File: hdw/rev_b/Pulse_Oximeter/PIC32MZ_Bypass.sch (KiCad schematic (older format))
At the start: 23 parts

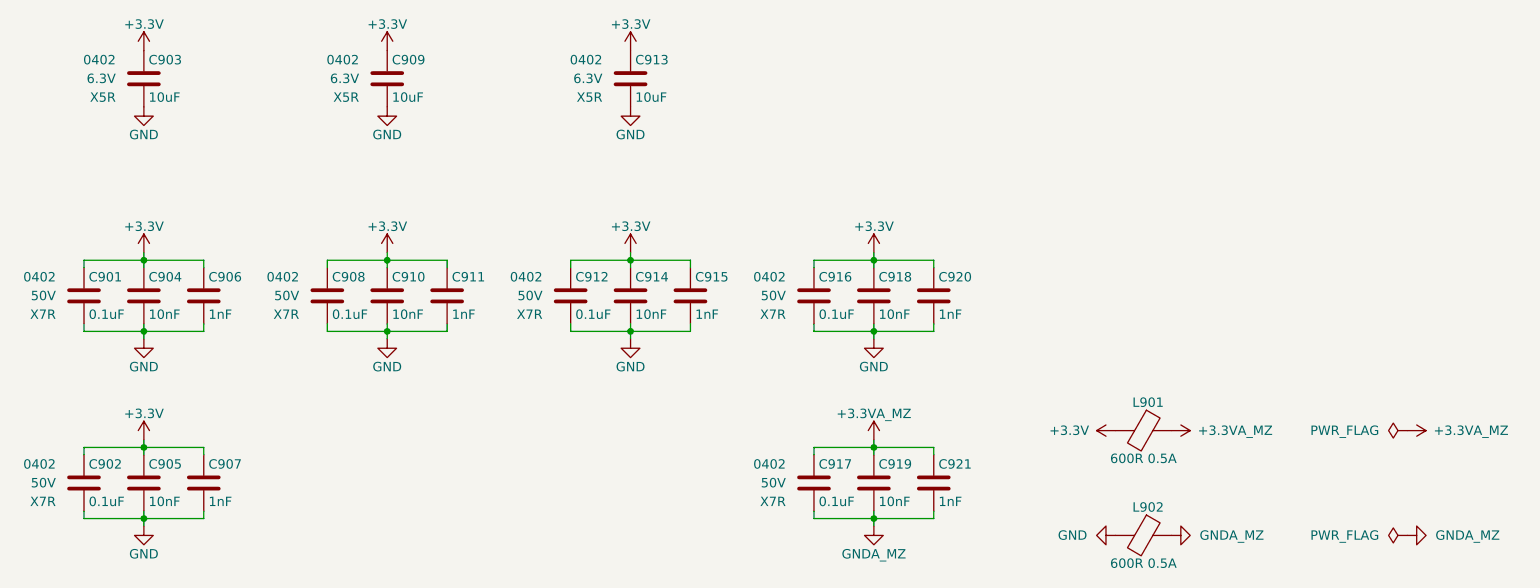
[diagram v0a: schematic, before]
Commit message: lots of rev b changes
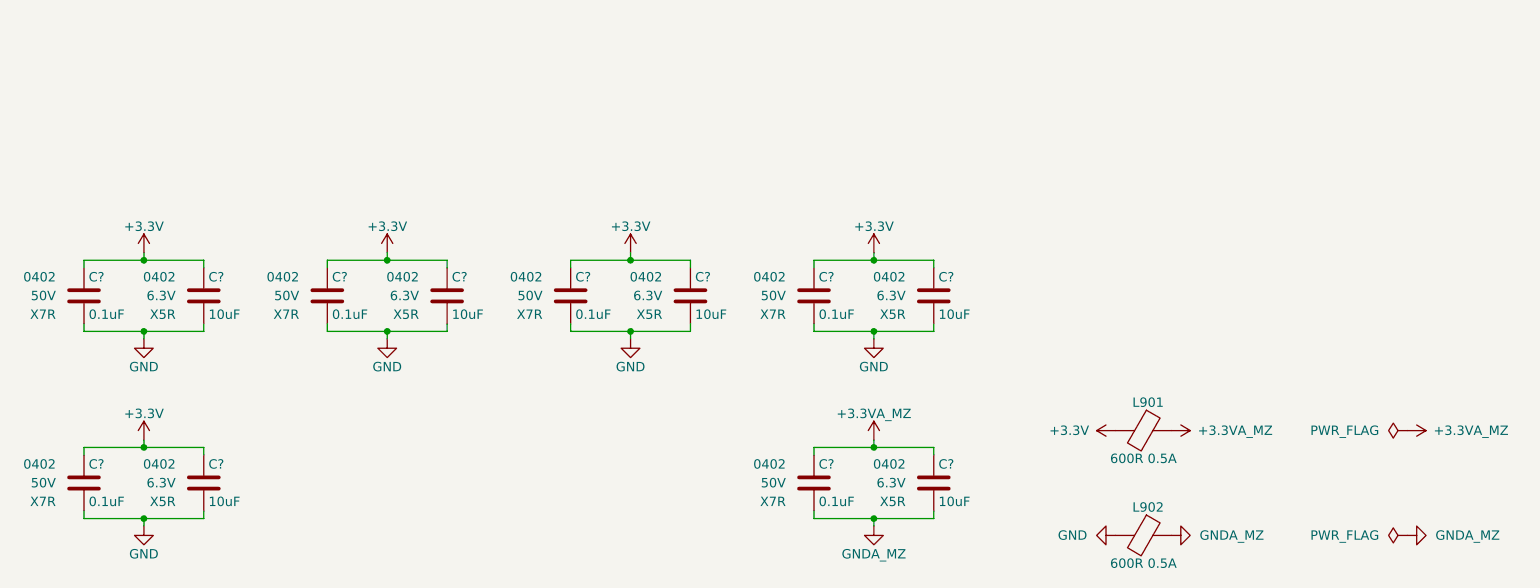
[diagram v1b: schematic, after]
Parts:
- removed C901, C902, C908, C912, C916, C917: 0.1uF, Capacitors_SMD:C_0402, symbol Custom_Library:C_Custom
- removed C903, C909, C913: 10uF, Capacitors_SMD:C_0402, symbol Custom_Library:C_Custom
- removed C904, C905, C910, C914, C918, C919: 10nF, Capacitors_SMD:C_0402, symbol Custom_Library:C_Custom
- removed C906, C907, C911, C915, C920, C921: 1nF, Capacitors_SMD:C_0402, symbol Custom_Library:C_Custom
- added C? (x6): 10uF, Capacitors_SMD:C_0402, symbol Custom_Library:C_Custom
- added C? (x6): 0.1uF, Capacitors_SMD:C_0402, symbol Custom_Library:C_Custom
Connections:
- net +3.3VA_MZ: now also C?.1, C?.1
- net +3V3: now also C?.1, C?.1, C?.1, C?.1, C?.1, C?.1, C?.1, C?.1, C?.1, C?.1
- net GND: now also C?.2, C?.2, C?.2, C?.2, C?.2, C?.2, C?.2, C?.2, C?.2, C?.2
- net GNDA_MZ: now also C?.2, C?.2

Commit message: changed all passives to 0402, cleared digikey pns
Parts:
- C? (x6): Digi-Key PN 490-13211-1-ND -> (none)
- C? (x6): Digi-Key PN 490-10701-1-ND -> (none)
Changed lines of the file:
@@
 F 5 "6.3V" H 3090 4400 50  0000 R CNN "Voltage"
 F 6 "X5R" H 3090 4300 50  0000 R CNN "Dielectric"
-F 7 "490-13211-1-ND" H 3240 4400 50  0001 C CNN "Digi-Key PN"
+F 7 "" H 3240 4400 50  0001 C CNN "Digi-Key PN"
 	1    3240 4400
 	1    0    0    -1
@@
 F 5 "50V" H 2450 4400 50  0000 R CNN "Voltage"
 F 6 "X7R" H 2450 4300 50  0000 R CNN "Dielectric"
-F 7 "490-10701-1-ND" H 3025 4900 60  0001 C CNN "Digi-Key PN"
+F 7 "" H 3025 4900 60  0001 C CNN "Digi-Key PN"
 	1    2600 4400
 	1    0    0    -1
@@
 F 5 "6.3V" H 3090 3400 50  0000 R CNN "Voltage"
 F 6 "X5R" H 3090 3300 50  0000 R CNN "Dielectric"
-F 7 "490-13211-1-ND" H 3240 3400 50  0001 C CNN "Digi-Key PN"
+F 7 "" H 3240 3400 50  0001 C CNN "Digi-Key PN"
 	1    3240 3400
 	1    0    0    -1
@@
 F 5 "50V" H 2450 3400 50  0000 R CNN "Voltage"
 F 6 "X7R" H 2450 3300 50  0000 R CNN "Dielectric"
-F 7 "490-10701-1-ND" H 3025 3900 60  0001 C CNN "Digi-Key PN"
+F 7 "" H 3025 3900 60  0001 C CNN "Digi-Key PN"
 	1    2600 3400
 	1    0    0    -1
@@
 F 5 "6.3V" H 4390 3400 50  0000 R CNN "Voltage"
 F 6 "X5R" H 4390 3300 50  0000 R CNN "Dielectric"
-F 7 "490-13211-1-ND" H 4540 3400 50  0001 C CNN "Digi-Key PN"
+F 7 "" H 4540 3400 50  0001 C CNN "Digi-Key PN"
 	1    4540 3400
 	1    0    0    -1
@@
 F 5 "50V" H 3750 3400 50  0000 R CNN "Voltage"
 F 6 "X7R" H 3750 3300 50  0000 R CNN "Dielectric"
-F 7 "490-10701-1-ND" H 4325 3900 60  0001 C CNN "Digi-Key PN"
+F 7 "" H 4325 3900 60  0001 C CNN "Digi-Key PN"
 	1    3900 3400
 	1    0    0    -1
@@
 F 5 "6.3V" H 5690 3400 50  0000 R CNN "Voltage"
 F 6 "X5R" H 5690 3300 50  0000 R CNN "Dielectric"
-F 7 "490-13211-1-ND" H 5840 3400 50  0001 C CNN "Digi-Key PN"
+F 7 "" H 5840 3400 50  0001 C CNN "Digi-Key PN"
 	1    5840 3400
 	1    0    0    -1
@@
 F 5 "50V" H 5050 3400 50  0000 R CNN "Voltage"
 F 6 "X7R" H 5050 3300 50  0000 R CNN "Dielectric"
-F 7 "490-10701-1-ND" H 5625 3900 60  0001 C CNN "Digi-Key PN"
+F 7 "" H 5625 3900 60  0001 C CNN "Digi-Key PN"
 	1    5200 3400
 	1    0    0    -1
@@
 F 5 "6.3V" H 6990 3400 50  0000 R CNN "Voltage"
 F 6 "X5R" H 6990 3300 50  0000 R CNN "Dielectric"
-F 7 "490-13211-1-ND" H 7140 3400 50  0001 C CNN "Digi-Key PN"
+F 7 "" H 7140 3400 50  0001 C CNN "Digi-Key PN"
 	1    7140 3400
 	1    0    0    -1
@@
 F 5 "50V" H 6350 3400 50  0000 R CNN "Voltage"
 F 6 "X7R" H 6350 3300 50  0000 R CNN "Dielectric"
-F 7 "490-10701-1-ND" H 6925 3900 60  0001 C CNN "Digi-Key PN"
+F 7 "" H 6925 3900 60  0001 C CNN "Digi-Key PN"
 	1    6500 3400
 	1    0    0    -1
@@
 F 5 "6.3V" H 6990 4400 50  0000 R CNN "Voltage"
 F 6 "X5R" H 6990 4300 50  0000 R CNN "Dielectric"
-F 7 "490-13211-1-ND" H 7140 4400 50  0001 C CNN "Digi-Key PN"
+F 7 "" H 7140 4400 50  0001 C CNN "Digi-Key PN"
 	1    7140 4400
 	1    0    0    -1
@@
 F 5 "50V" H 6350 4400 50  0000 R CNN "Voltage"
 F 6 "X7R" H 6350 4300 50  0000 R CNN "Dielectric"
-F 7 "490-10701-1-ND" H 6925 4900 60  0001 C CNN "Digi-Key PN"
+F 7 "" H 6925 4900 60  0001 C CNN "Digi-Key PN"
 	1    6500 4400
 	1    0    0    -1
